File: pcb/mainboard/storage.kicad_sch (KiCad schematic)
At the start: 46 parts, among them J401 MICRO_SD(TFC-WPAPR-08), J402 Hard Drive, J403 Optical Drive, U401 ASM1061, Y401 20MHz

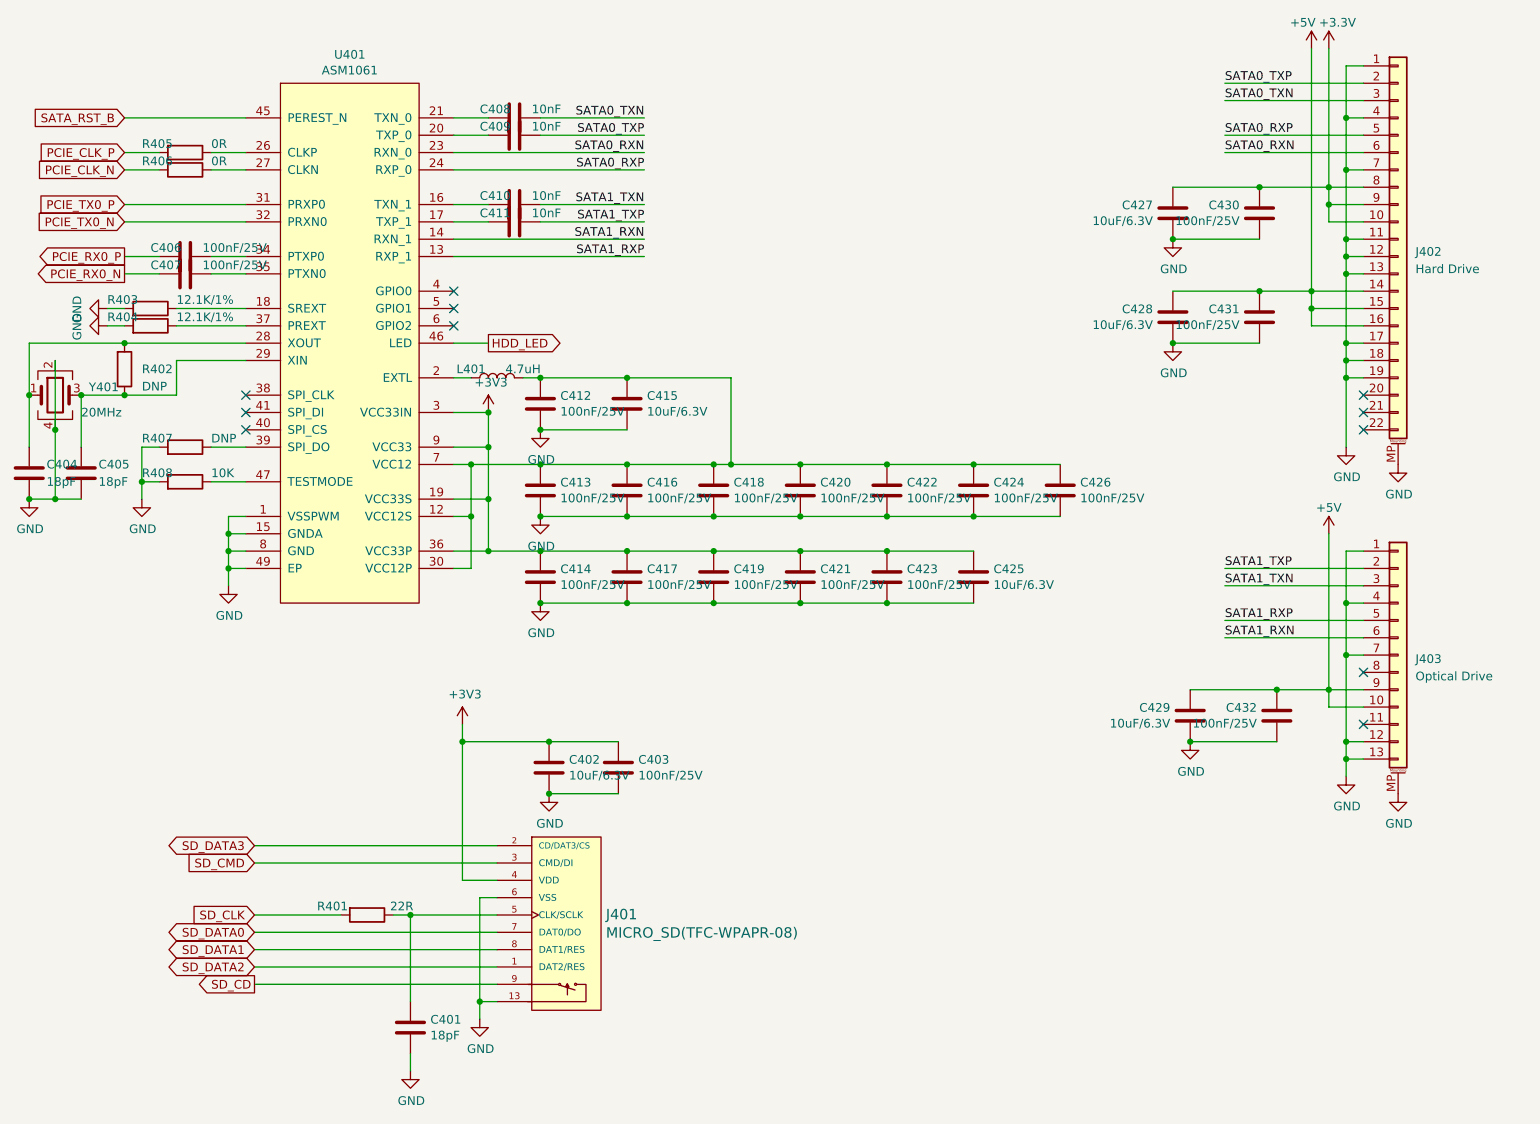
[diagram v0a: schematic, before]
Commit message: pcb: r0.1 mb routing done
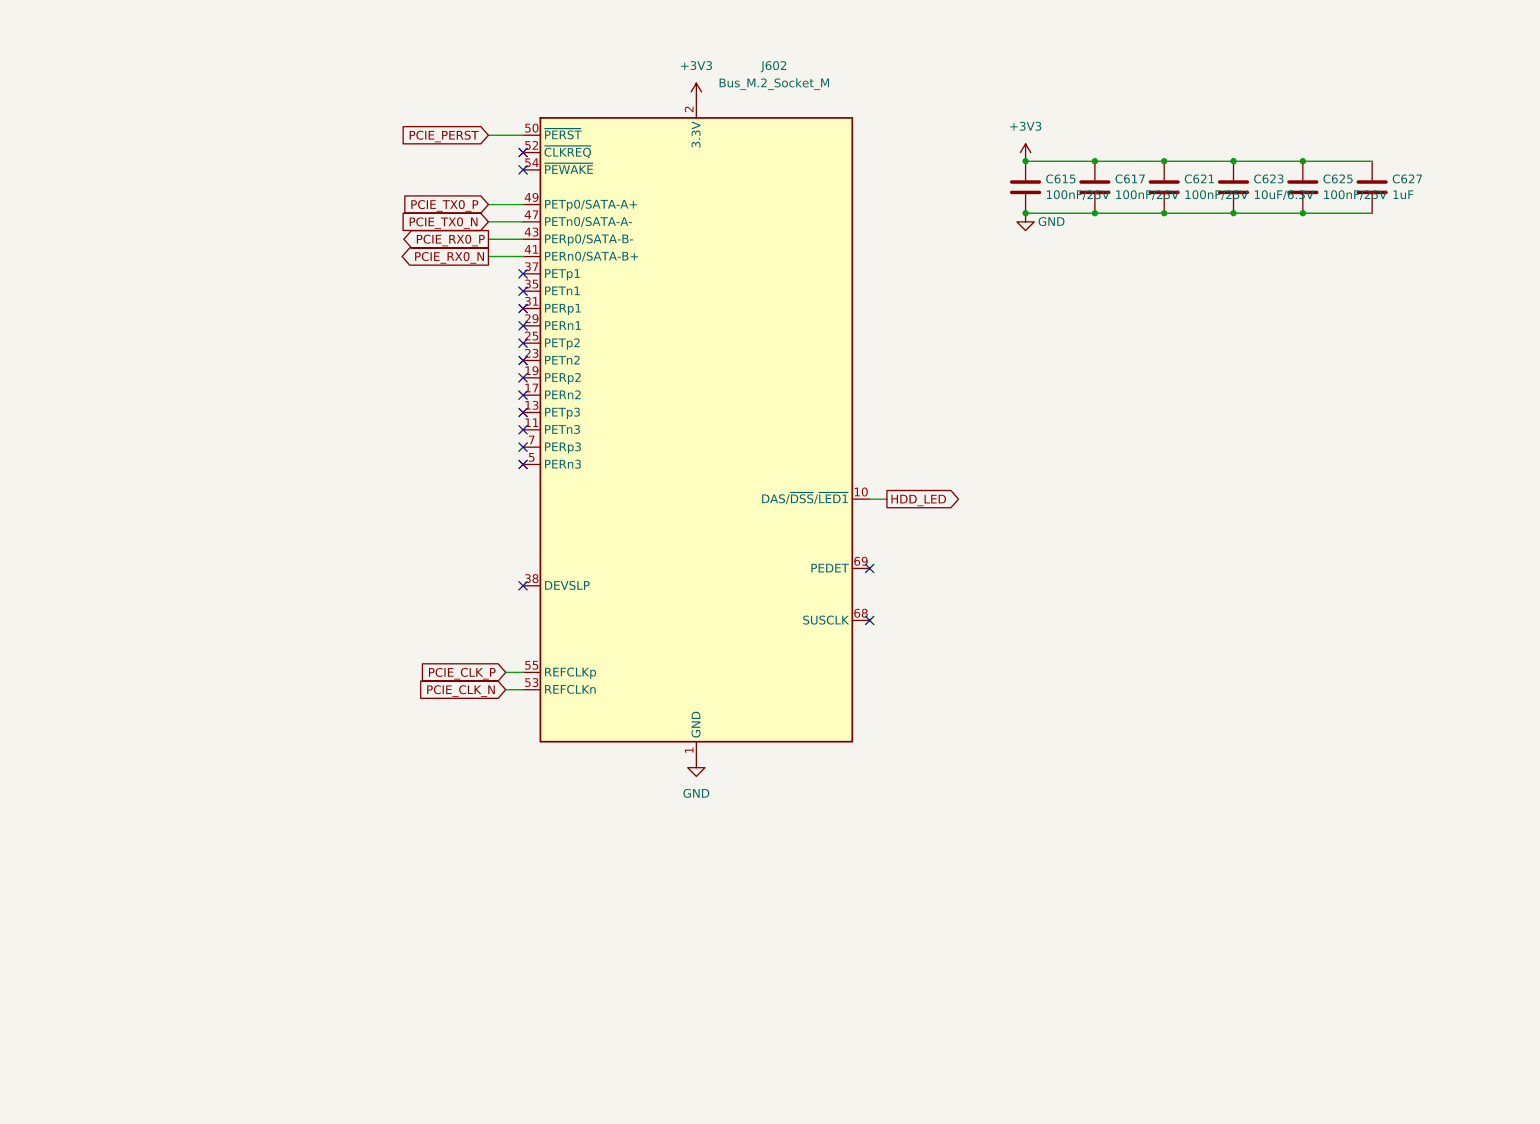
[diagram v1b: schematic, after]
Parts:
- removed C401, C404, C405: 18pF, Capacitor_SMD:C_0402_1005Metric, symbol Device:C
- removed C402, C415, C425, C427, C428, C429: 10uF/6.3V, Capacitor_SMD:C_0603_1608Metric, symbol Device:C
- removed C403, C406, C407, C412, C413, C414, C416, C417, C418, C419, C420, C421, C422, C423, C424, C426, C430, C431, C432: 100nF/25V, Capacitor_SMD:C_0402_1005Metric, symbol Device:C
- removed C408, C409, C410, C411: 10nF, Capacitor_SMD:C_0402_1005Metric, symbol Device:C
- removed J401: MICRO_SD(TFC-WPAPR-08), footprints:TFC-WPAPR-08, symbol symbols:MICRO_SD(TFC-WPAPR-08)
- removed J402: Hard Drive, footprints:TE_2023246-2, symbol Connector_Generic_MountingPin:Conn_01x22_MountingPin
- removed J403: Optical Drive, footprints:TE_1735413-1, symbol Connector_Generic_MountingPin:Conn_01x13_MountingPin
- removed L401: 4.7uH, footprints:L_1212, symbol Device:L
- removed R401: 22R, Resistor_SMD:R_0402_1005Metric, symbol Device:R
- removed R402, R407: DNP, Resistor_SMD:R_0402_1005Metric, symbol Device:R
- removed R403, R404: 12.1K/1%, Resistor_SMD:R_0402_1005Metric, symbol Device:R
- removed R405, R406: 0R, Resistor_SMD:R_0402_1005Metric, symbol Device:R
- removed R408: 10K, Resistor_SMD:R_0402_1005Metric, symbol Device:R
- removed U401: ASM1061, Package_DFN_QFN:QFN-48-1EP_7x7mm_P0.5mm_EP5.15x5.15mm_ThermalVias, symbol symbols:ASM1061
- removed Y401: 20MHz, Crystal:Crystal_SMD_3225-4Pin_3.2x2.5mm, symbol Device:Crystal_GND24
- added C615, C617, C621, C625: 100nF/25V, Capacitor_SMD:C_0402_1005Metric, symbol Device:C
- added C623: 10uF/6.3V, Capacitor_SMD:C_0603_1608Metric, symbol Device:C
- added C627: 1uF, Capacitor_SMD:C_0402_1005Metric, symbol Device:C
- added J602: Bus_M.2_Socket_M, footprints:M2_MKEY, symbol Connector:Bus_M.2_Socket_M
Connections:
- net +3V3: now also C615.1, C617.1, C621.1, C623.1, C625.1, C627.1, J602.12 (3.3V), J602.14 (3.3V), J602.16 (3.3V), J602.18 (3.3V), J602.2 (3.3V), J602.4 (3.3V), J602.70 (3.3V), J602.72 (3.3V), J602.74 (3.3V)
- net GND: now also C615.2, C617.2, C621.2, C623.2, C625.2, C627.2, J602.1 (GND), J602.15 (GND), J602.21 (GND), J602.27 (GND), J602.3 (GND), J602.33 (GND), J602.39 (GND), J602.45 (GND), J602.51 (GND), J602.57 (GND), J602.71 (GND), J602.73 (GND), J602.75 (GND), J602.9 (GND)
- net HDD_LED: now also J602.10 (DAS/~{DSS}/~{LED1})
- net PCIE_CLK_N: now also J602.53 (REFCLKn)
- net PCIE_CLK_P: now also J602.55 (REFCLKp)
- net PCIE_RX0_N: now also J602.41 (PERn0/SATA-B+)
- net PCIE_RX0_P: now also J602.43 (PERp0/SATA-B-)
- net PCIE_TX0_N: now also J602.47 (PETn0/SATA-A-)
- net PCIE_TX0_P: now also J602.49 (PETp0/SATA-A+)
- new net PCIE_PERST: J602.50 (~{PERST})
- no-connect marks 11 -> 17
